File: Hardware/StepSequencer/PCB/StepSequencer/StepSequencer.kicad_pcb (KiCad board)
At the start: 2 copper layers, 54 parts, among them J1 Conn_01x04_Male, SW1 SW_DIP_x01, SW10 SW_DIP_x01, SW11 SW_DIP_x01, SW12 SW_DIP_x01, SW13 SW_DIP_x01, SW14 SW_DIP_x01, SW15 SW_DIP_x01, SW16 SW_DIP_x01, SW17 SW_DIP_x01, SW18 SW_DIP_x01, SW19 SW_DIP_x01, SW2 SW_DIP_x01, SW20 SW_DIP_x01, SW21 SW_DIP_x01, SW22 SW_DIP_x01, SW23 SW_DIP_x01, SW3 SW_DIP_x01, SW4 SW_DIP_x01, SW5 SW_DIP_x01, SW6 SW_DIP_x01, SW7 SW_DIP_x01, SW8 SW_DIP_x01, SW9 SW_DIP_x01, U1 MCP23017_SP

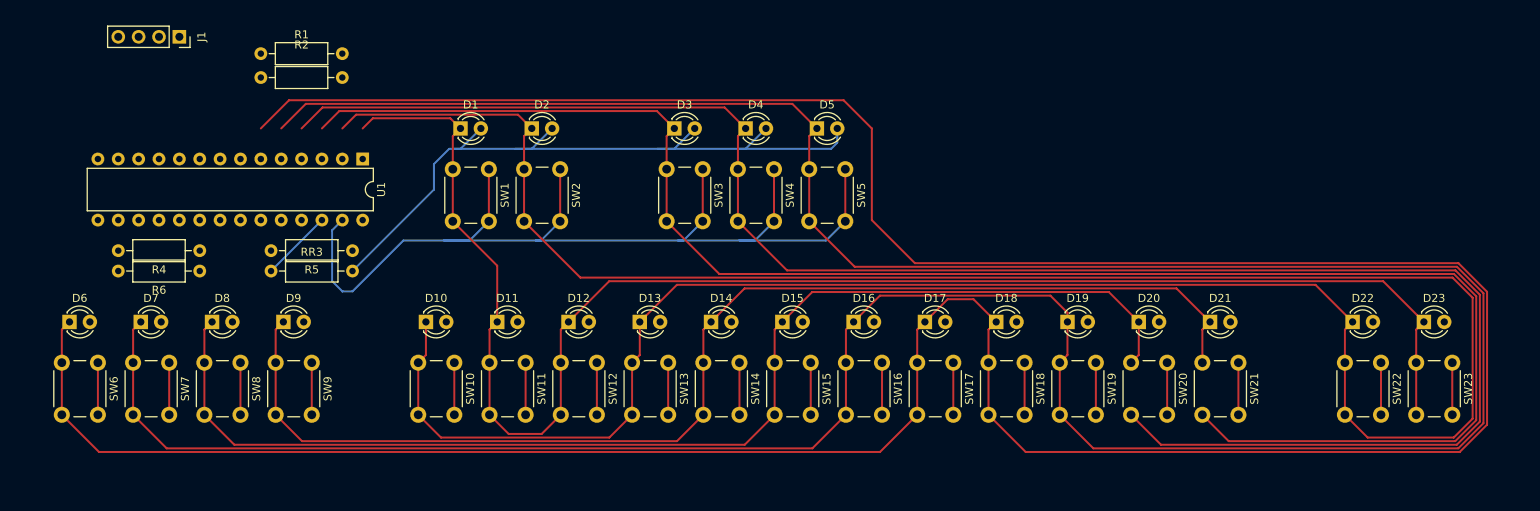
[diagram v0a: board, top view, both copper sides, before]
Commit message: Initial test for StepSequencer
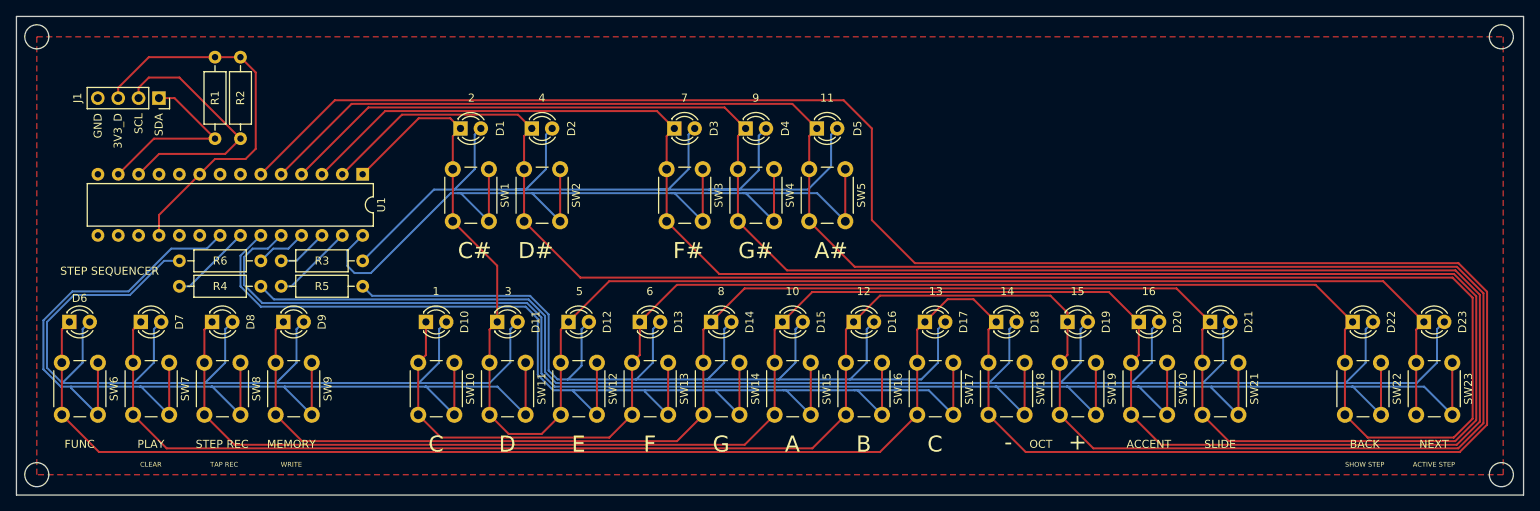
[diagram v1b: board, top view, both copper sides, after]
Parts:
- moved R1 12.0 mm to (69.2, 100.4), turned to 90 degrees
- moved R5 9.94 mm to (77.5, 118.8), turned to 0 degrees
- moved J1 8.06 mm to (62.2, 95.3)
- moved R2 8.03 mm to (72.4, 100.4), turned to 90 degrees
- moved R6 7.73 mm to (74.9, 115.6)
- moved R4 5.12 mm to (64.8, 118.8), turned to 0 degrees
- moved U1 1.91 mm to (87.6, 104.8)
- moved R3 1.80 mm to (77.5, 115.6)
- renumbered RR3 to R3
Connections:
- R5 pad 1: GPA7 -> GPA6
- R6 pad 1: GPA3 -> GPA4
- SW1 pad 1: GPA6 -> GPA7
- SW10 pad 1: GPA2 -> GPA0
- SW11 pad 1: GPA2 -> GPA0
- SW12 pad 1: GPA4 -> GPA2
- SW13 pad 1: GPA4 -> GPA2
- SW14 pad 1: GPA4 -> GPA2
- SW15 pad 1: GPA4 -> GPA2
- SW16 pad 1: GPA4 -> GPA2
- SW17 pad 1: GPA4 -> GPA2
- SW18 pad 1: GPA0 -> GPA3
- SW19 pad 1: GPA0 -> GPA3
- SW2 pad 1: GPA6 -> GPA7
- SW20 pad 1: GPA0 -> GPA3
- SW21 pad 1: GPA0 -> GPA3
- SW22 pad 1: GPA0 -> GPA3
- SW23 pad 1: GPA0 -> GPA3
- SW3 pad 1: GPA6 -> GPA7
- SW4 pad 1: GPA6 -> GPA7
- SW5 pad 1: GPA6 -> GPA7
- SW6 pad 1: GPA2 -> GPA0
- SW7 pad 1: GPA2 -> GPA0
- SW8 pad 1: GPA2 -> GPA0
- SW9 pad 1: GPA2 -> GPA0
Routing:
- net GPA3: track 0.00 -> 234.9 mm
- net Net-(D18-Pad2): track 0.00 -> 207.5 mm
- net Net-(D10-Pad2): track 0.00 -> 136.3 mm
- net GPA2: track 39.0 -> 168.2 mm
- net Net-(D12-Pad2): track 0.00 -> 128.9 mm
- net GPA7: track 0.00 -> 126.7 mm
- net GPA0: track 39.0 -> 159.1 mm
- net GPA6: track 129.4 -> 10.3 mm
- net 3V3_D: track 0.00 -> 49.0 mm
- net GPA4: track 39.0 -> 6.42 mm
- net SCL: track 0.00 -> 32.2 mm
- net SDA: track 0.00 -> 23.0 mm
- net Net-(D1-Pad2): track 91.2 -> 111.2 mm
- net GPA1: track 0.00 -> 10.3 mm
- net GPB3: track 379.1 -> 388.0 mm
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- added copper zone on F.Cu, net GND
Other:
- board outline added: 188 x 59.7 mm
- board text added: "+"
- board text added: "-"
- board text added: "1"
- board text added: "10"
- board text added: "11"
- board text added: "12"
- board text added: "13"
- board text added: "14"
- board text added: "15"
- board text added: "16"
- board text added: "2"
- board text added: "3"
- board text added: "3V3_D"
- board text added: "4"
- board text added: "5"
- board text added: "6"
- board text added: "7"
- board text added: "8"
- board text added: "9"
- board text added: "A"
- board text added: "A#"
- board text added: "ACCENT"
- board text added: "ACTIVE STEP"
- board text added: "B"
- board text added: "BACK"
- board text added: "C"
- board text added: "C#"
- board text added: "CLEAR"
- board text added: "D"
- board text added: "D#"
- board text added: "E"
- board text added: "F"
- board text added: "F#"
- board text added: "FUNC"
- board text added: "G"
- board text added: "G#"
- board text added: "GND"
- board text added: "MEMORY"
- board text added: "NEXT"
- board text added: "OCT"
- board text added: "PLAY"
- board text added: "SCL"
- board text added: "SDA"
- board text added: "SHOW STEP"
- board text added: "SLIDE"
- board text added: "STEP REC"
- board text added: "STEP SEQUENCER"
- board text added: "TAP REC"
- board text added: "WRITE"
